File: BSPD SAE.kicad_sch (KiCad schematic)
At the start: 37 parts, among them U1 LTC6994xS6-2, U3 TLV1824, U4 TLV1824

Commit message: autosave 2026-10-04 20:27:48
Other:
- note added: "Delay block"
- moved on the sheet: C11, C9, R1, R2, R3, R44, R45, R46, U1

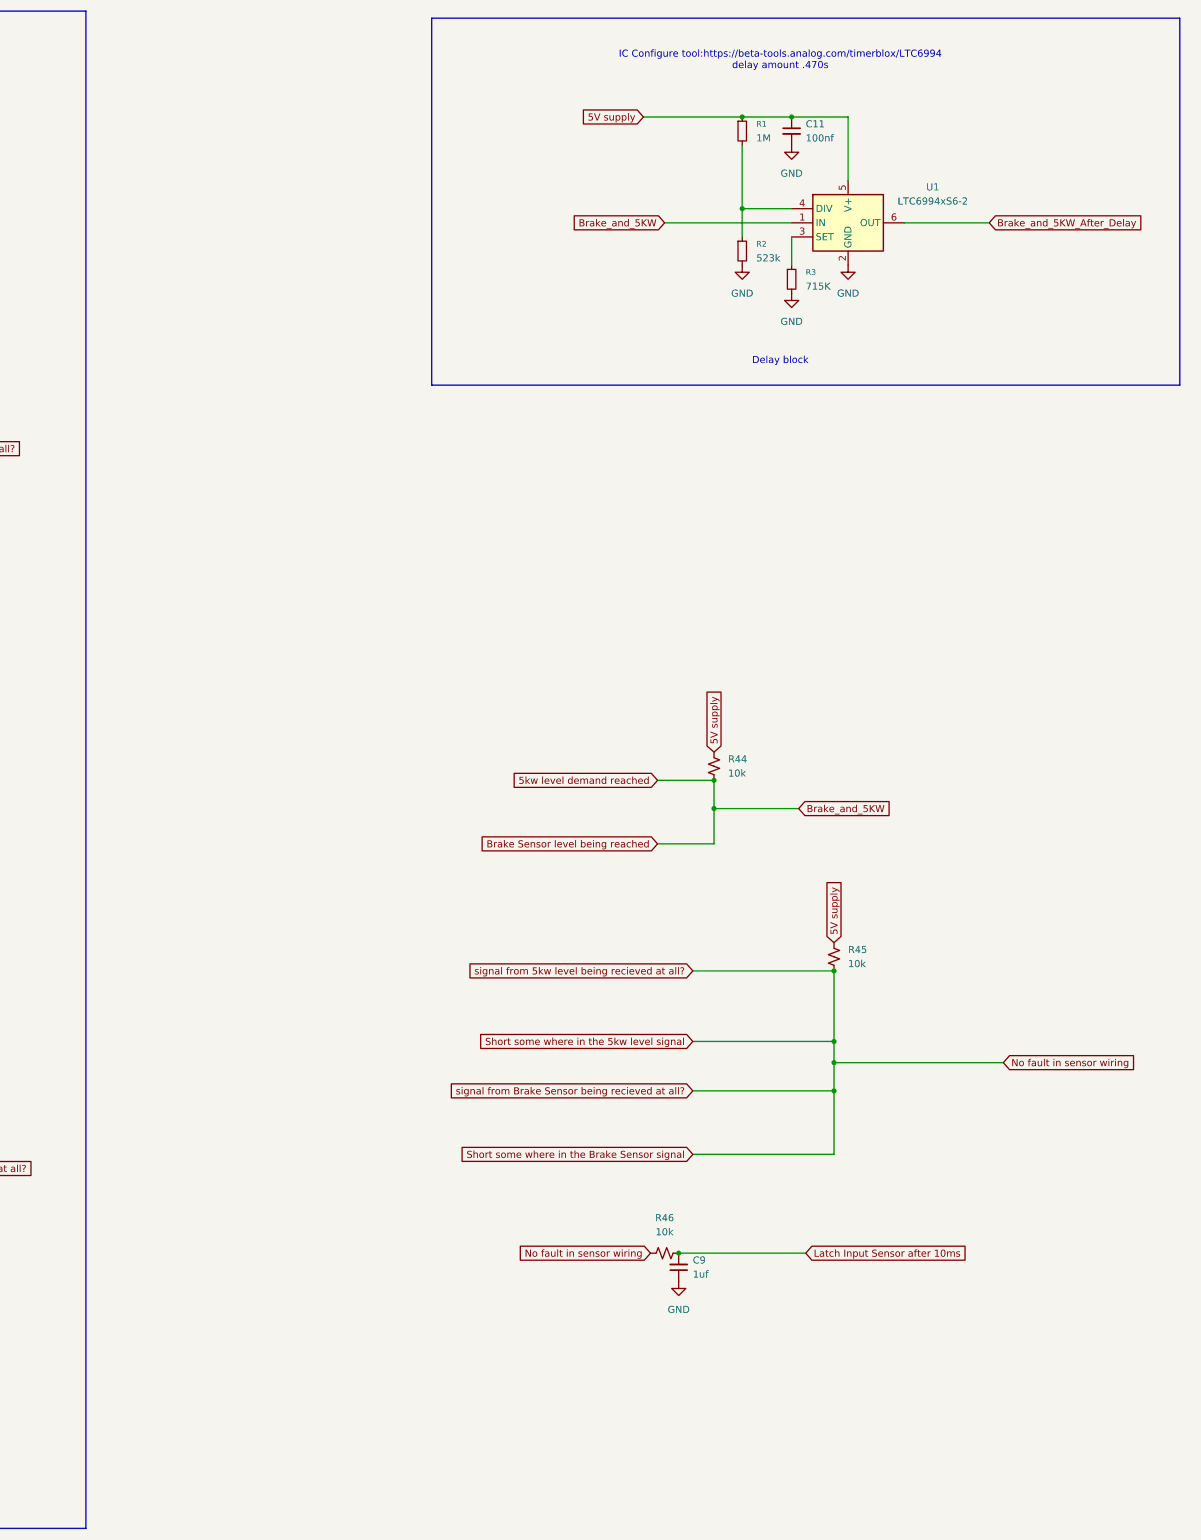
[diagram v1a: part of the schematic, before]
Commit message: autosave 2026-10-04 21:16:58
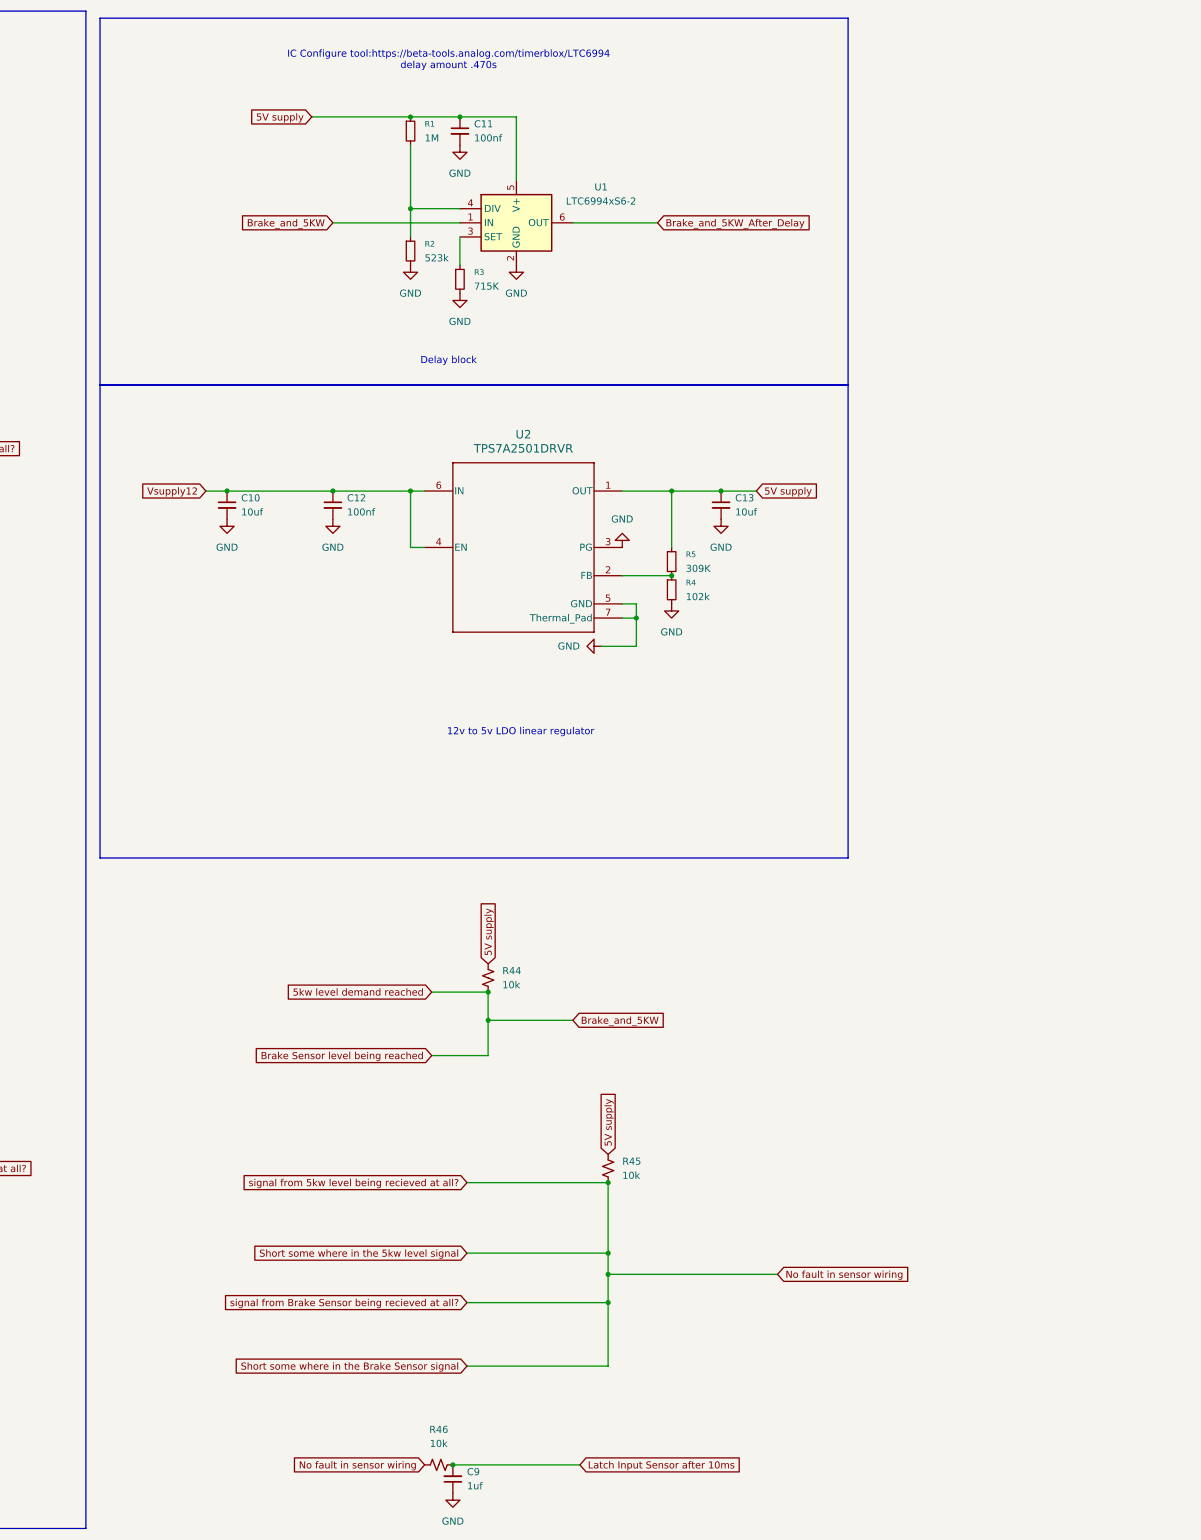
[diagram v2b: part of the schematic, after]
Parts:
- added C10, C13: 10uf, Capacitor_SMD:C_0805_2012Metric, symbol Device:C_Small
- added C12: 100nf, Capacitor_SMD:C_0805_2012Metric, symbol Device:C_Small
- added R4: 102k, Resistor_SMD:R_0805_2012Metric, symbol Device:R_Small
- added R5: 309K, Resistor_SMD:R_0805_2012Metric, symbol Device:R_Small
- added U2: TPS7A2501DRVR, DRV0006A-IPC_A, symbol 2026-10-05_03-25-03:TPS7A2501DRVR
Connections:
- net 5V supply: now also C13.1, R5.1, U2.1 (OUT)
- net GND: now also C10.2, C12.2, C13.2, R4.2, U2.3 (PG), U2.5 (GND), U2.7 (Thermal_Pad)
- net Vsupply12: now also C10.1, C12.1, U2.4 (EN), U2.6 (IN)
- new net: R4.1, R5.2, U2.2 (FB)
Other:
- note added: "12v to 5v LDO linear regulator"
- moved on the sheet: C11, C9, R1, R2, R3, R44, R45, R46, U1
